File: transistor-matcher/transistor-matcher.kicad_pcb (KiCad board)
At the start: 2 copper layers, 39.4 x 82.6 mm, 14 parts, among them J1 V+, J2 GND, J3 V-, J4 DMM1, J5 Conn_01x05_Female, J6 Conn_01x05_Female, J7 DMM2, SW1 SW_DPDT_x2

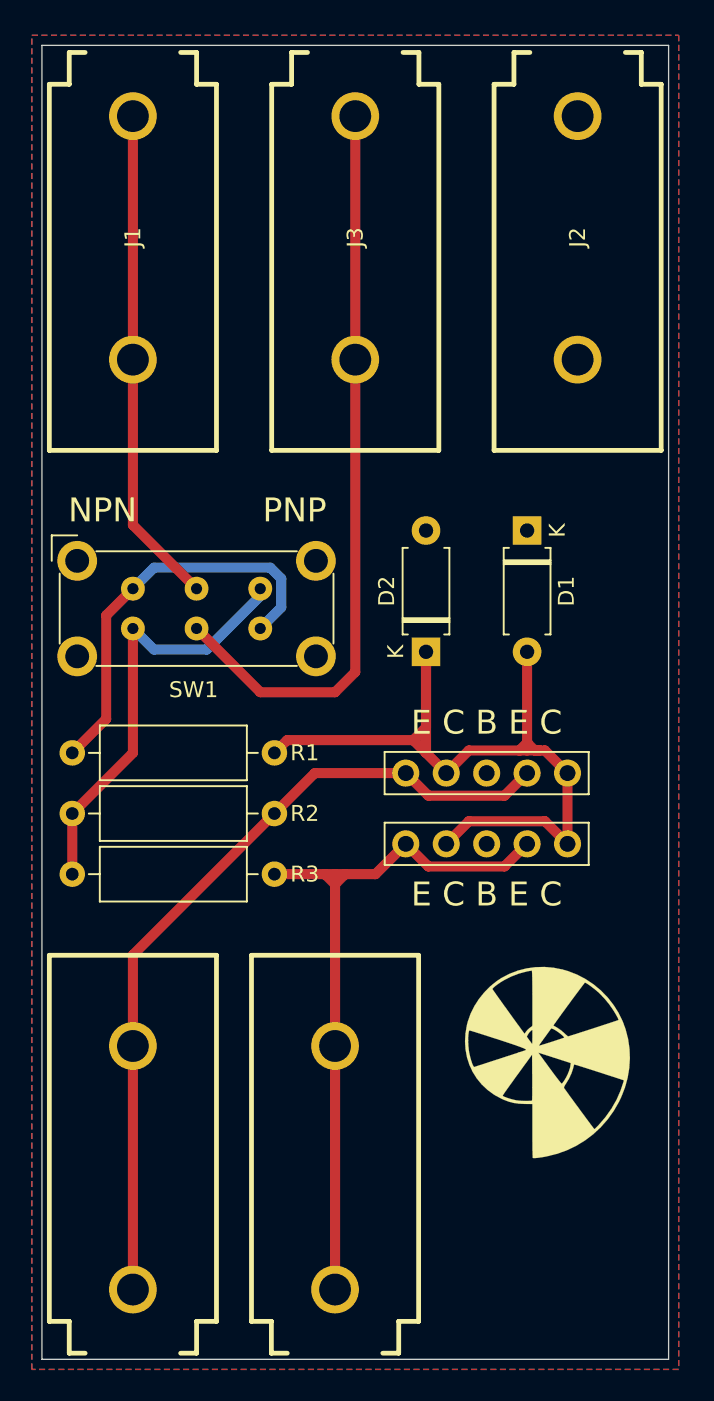
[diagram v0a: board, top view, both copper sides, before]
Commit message: Updating ordered boards
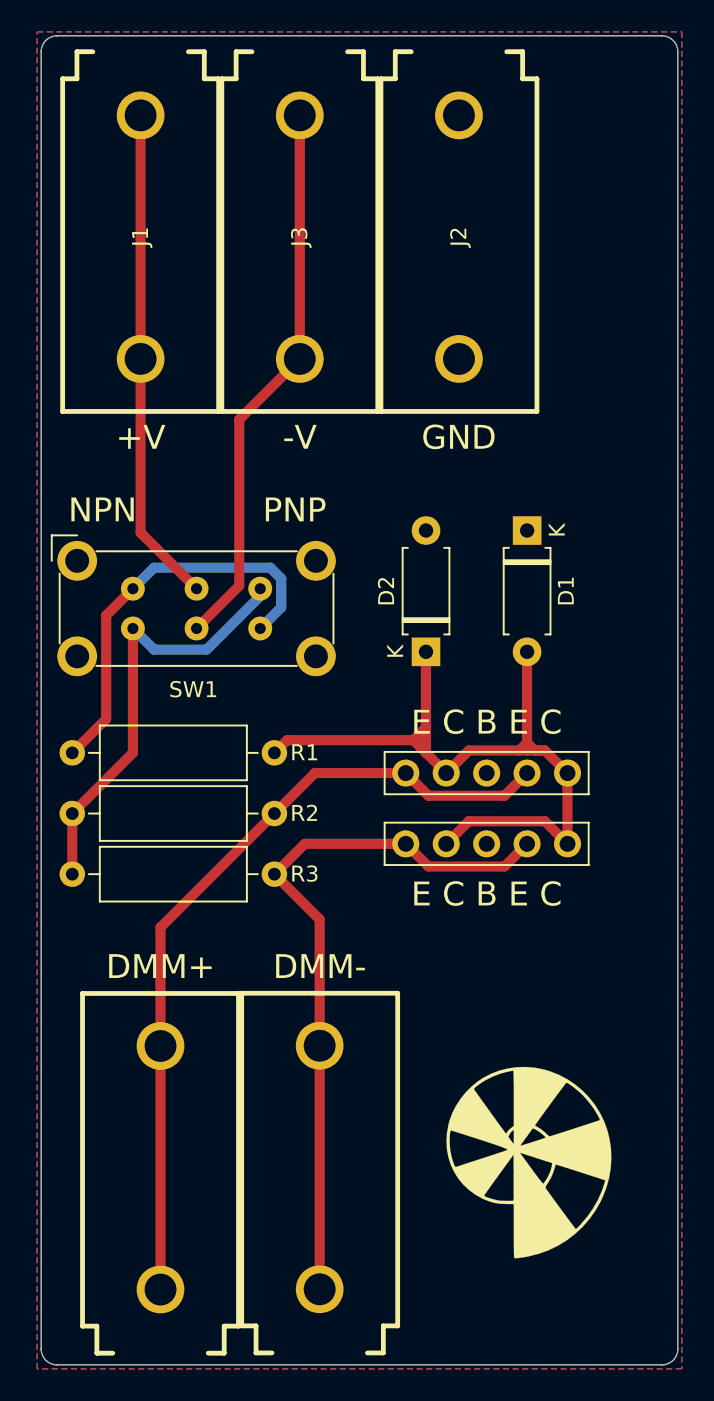
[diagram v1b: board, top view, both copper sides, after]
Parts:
- moved J2 7.46 mm to (108.8, 42.5)
- moved H1 6.39 mm to (112.5, 107.2)
- moved J3 3.49 mm to (98.8, 42.5)
- moved J4 1.73 mm to (90.0, 116.3)
- moved J7 0.97 mm to (100.0, 116.2)
- moved J1 0.49 mm to (88.8, 42.5)
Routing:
- net Net-(J3-Pad1): track 47.1 -> 34.9 mm
- net Net-(J4-Pad1): track 51.7 -> 51.0 mm
- net Net-(J6-Pad2): track 45.7 -> 45.1 mm
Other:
- board size 39.4 x 82.6 mm -> 40 x 83.5 mm
- board text added: "+V"
- board text added: "-V"
- board text added: "DMM+"
- board text added: "DMM-"
- board text added: "GND"
